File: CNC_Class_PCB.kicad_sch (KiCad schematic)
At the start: 16 parts, among them Q2 2N3904, U1 ICM7555xB

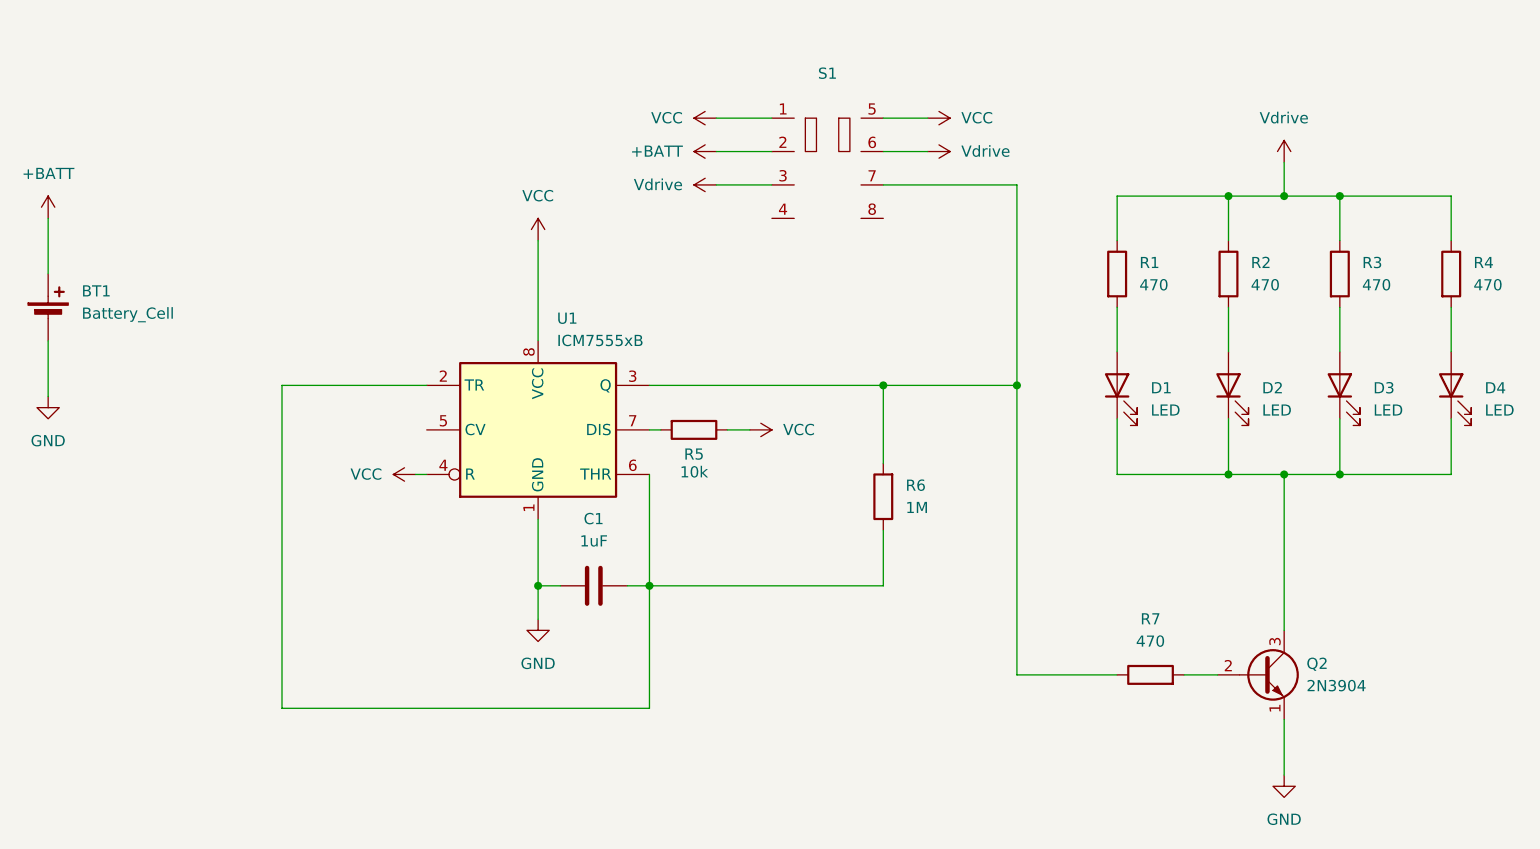
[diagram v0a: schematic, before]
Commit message: smol
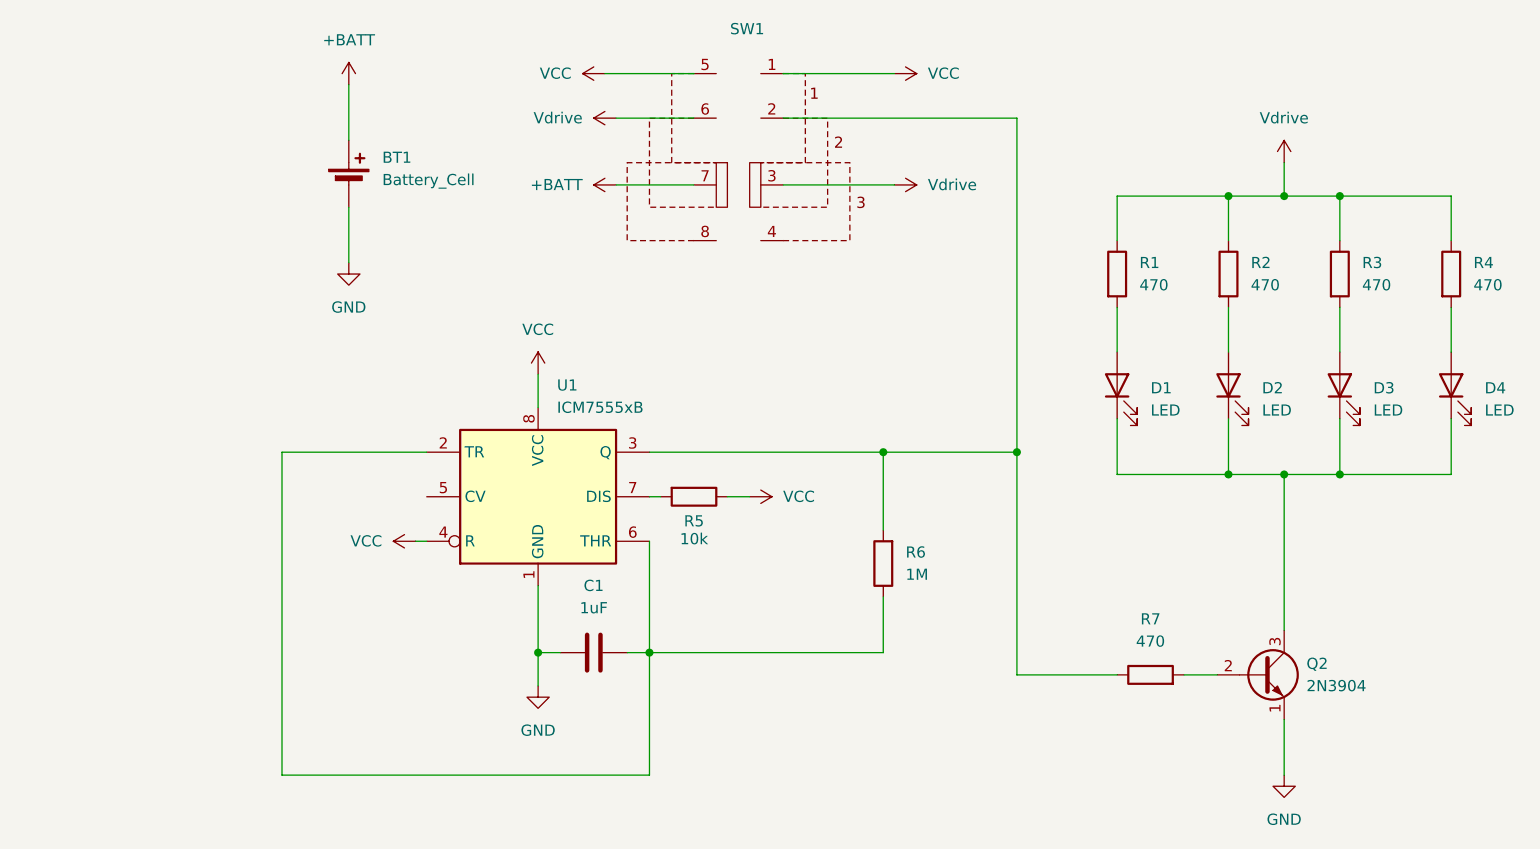
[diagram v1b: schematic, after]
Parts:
- removed S1: ~, My_Library:OS203013MT6QN1, symbol My_Library:DP3T_Slide
- added SW1: ~, My_Library:SLW-133538-2A-SMT-TR, symbol My_Library:DP3T
- BT1: footprint My_Library:BH-25C-1 -> My_Library:BAT-HLD-003-SMT
- R1, R2, R3, R4: footprint Resistor_THT:R_Axial_DIN0207_L6.3mm_D2.5mm_P15.24mm_Horizontal -> Resistor_THT:R_Axial_DIN0207_L6.3mm_D2.5mm_P10.16mm_Horizontal
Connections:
- net +BATT: now also SW1.7
- net VCC: now also SW1.1, SW1.5
- net Vdrive: now also SW1.3, SW1.6
- net at R6.2, R7.1, U1.3 (Q): now also SW1.2
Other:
- moved on the sheet: BT1, C1, R5, R6, U1
